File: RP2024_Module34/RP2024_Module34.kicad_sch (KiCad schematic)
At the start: 44 parts, among them J1 USB_C_Receptacle_USB2.0, J3 Conn_02x15_Odd_Even, U1 XC6206PxxxMR-Regulator_Linear, U2 PRTR5V0U2X, U3 W25Q128JVS, U4 RP2040, U5 74LVC1T45, Y1 12Mhz

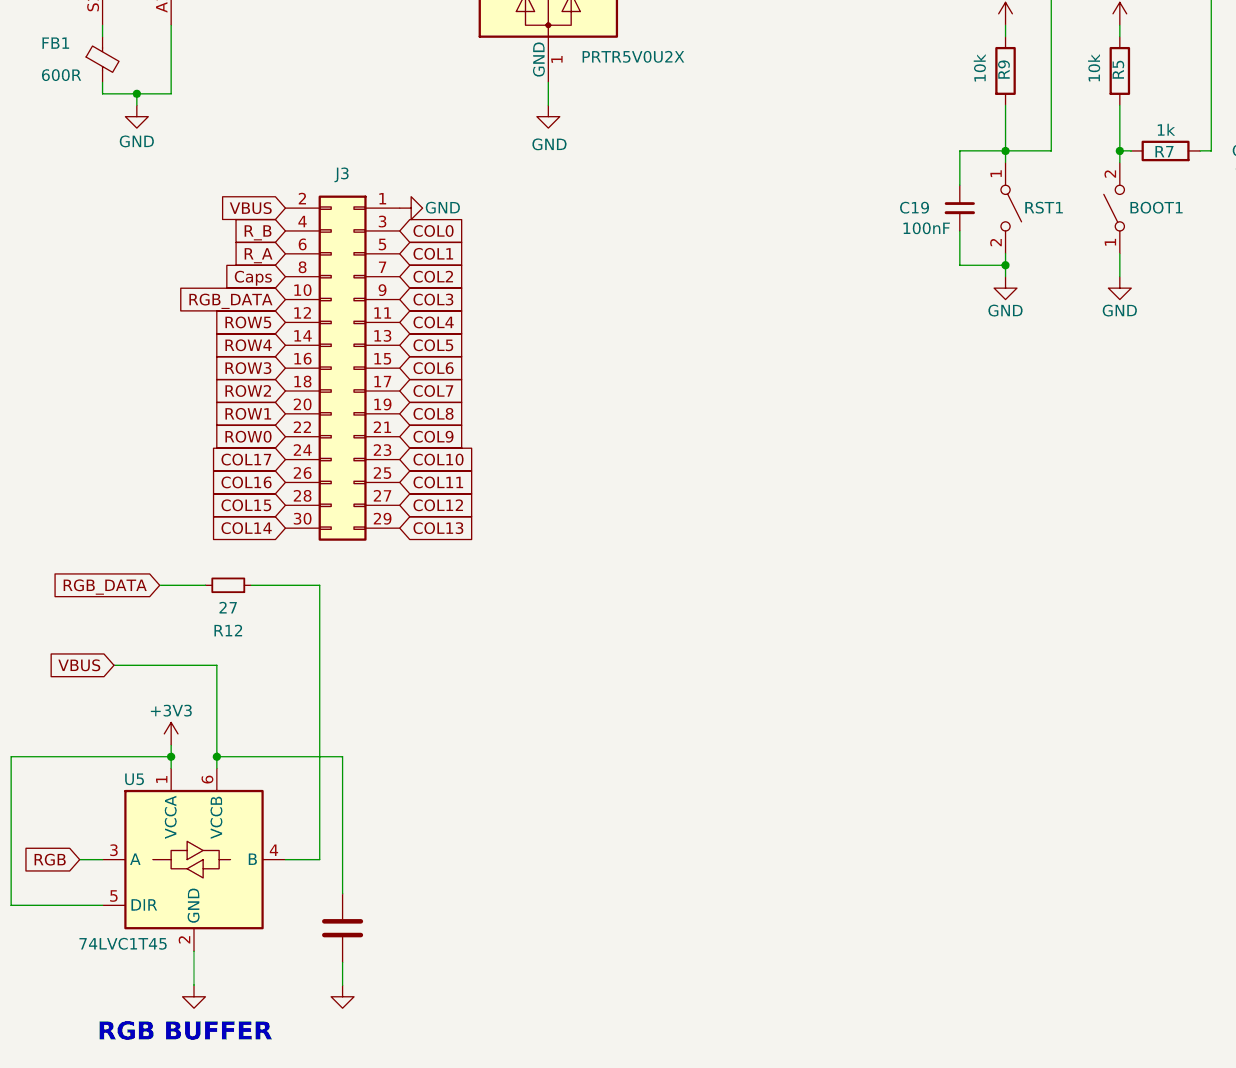
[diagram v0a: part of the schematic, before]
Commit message: Add files via upload
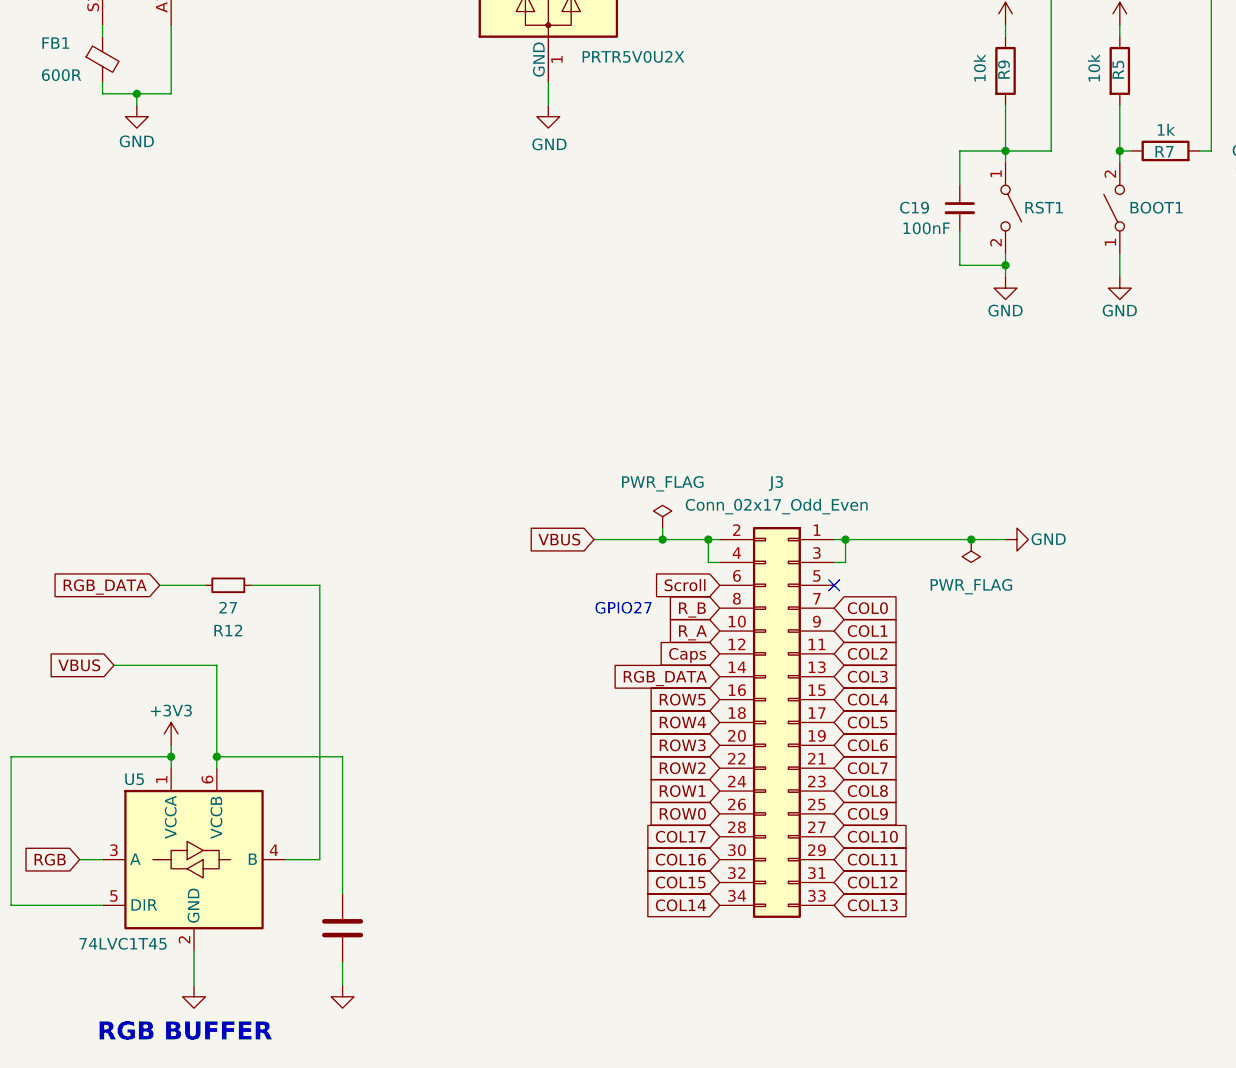
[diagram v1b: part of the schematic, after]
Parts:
- removed J3: Conn_02x15_Odd_Even, MyConnectors:IDC_2X15_1.27MM, symbol Connector_Generic:Conn_02x15_Odd_Even
- added J3: Conn_02x17_Odd_Even, MyConnectors:IDC_2X17_1.27MM, symbol Connector_Generic:Conn_02x17_Odd_Even
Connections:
- net COL0: now also J3.7 (Pin_7)
- net COL1: now also J3.9 (Pin_9)
- net COL10: now also J3.27 (Pin_27)
- net COL11: now also J3.29 (Pin_29)
- net COL12: now also J3.31 (Pin_31)
- net COL13: now also J3.33 (Pin_33)
- net COL14: now also J3.34 (Pin_34)
- net COL15: now also J3.32 (Pin_32)
- net COL16: now also J3.30 (Pin_30)
- net COL17: now also J3.28 (Pin_28)
- net COL2: now also J3.11 (Pin_11)
- net COL3: now also J3.13 (Pin_13)
- net COL4: now also J3.15 (Pin_15)
- net COL5: now also J3.17 (Pin_17)
- net COL6: now also J3.19 (Pin_19)
- net COL7: now also J3.21 (Pin_21)
- net COL8: now also J3.23 (Pin_23)
- net COL9: now also J3.25 (Pin_25)
- net Caps: now also J3.12 (Pin_12)
- net GND: now also J3.1 (Pin_1), J3.3 (Pin_3)
- net RGB_DATA: now also J3.14 (Pin_14)
- net ROW0: now also J3.26 (Pin_26)
- net ROW1: now also J3.24 (Pin_24)
- net ROW2: now also J3.22 (Pin_22)
- net ROW3: now also J3.20 (Pin_20)
- net ROW4: now also J3.18 (Pin_18)
- net ROW5: now also J3.16 (Pin_16)
- net R_A: now also J3.10 (Pin_10)
- net R_B: now also J3.8 (Pin_8)
- net VBUS: now also J3.2 (Pin_2), J3.4 (Pin_4)
- new net Scroll: J3.6 (Pin_6)
- no-connect marks 5 -> 6
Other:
- note added: "GPIO27"
